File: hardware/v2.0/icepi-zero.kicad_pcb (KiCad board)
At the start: 4 copper layers, 65 x 30 mm, 208 parts, among them IC1 IS42S16160J-6BLI, IC2 LTC2256CUJ-12#PBF, IC4 LTC2622IMS8#PBF, J1 Conn_02x20_Counter_Clockwise, J2 GPDI_C_1.3, J3 USB_C_Receptacle_USB2.0_14P, J4 USB_C_Receptacle_USB2.0_14P, J5 USB_C_Receptacle_USB2.0_14P, J6 Micro_SD_Card_Det2, J7 RSP-122811-01, J8 BM04B-ACHSS-A-GAN-TFLFSN, SW1 SW_Push, SW2 SW_Push, U1 ECP5U-25F-CABGA256, U10 TPD2EUSB30A, U11 LT1993CUD-2_PBF, U12 W25Q128JVS, U13 TCR5FM50A, U2 LTC3407AEDD-2_PBF, U3 TLV62569DBV, U5 TCR5FM18A, U6 PCA9306DC1, U7 TPD2EUSB30A, U8 TPD2EUSB30A, U9 FT231XQ, Y1 SG-8018CG 50.000000MHz, Y2 SG-8018CG 25.000000MHz

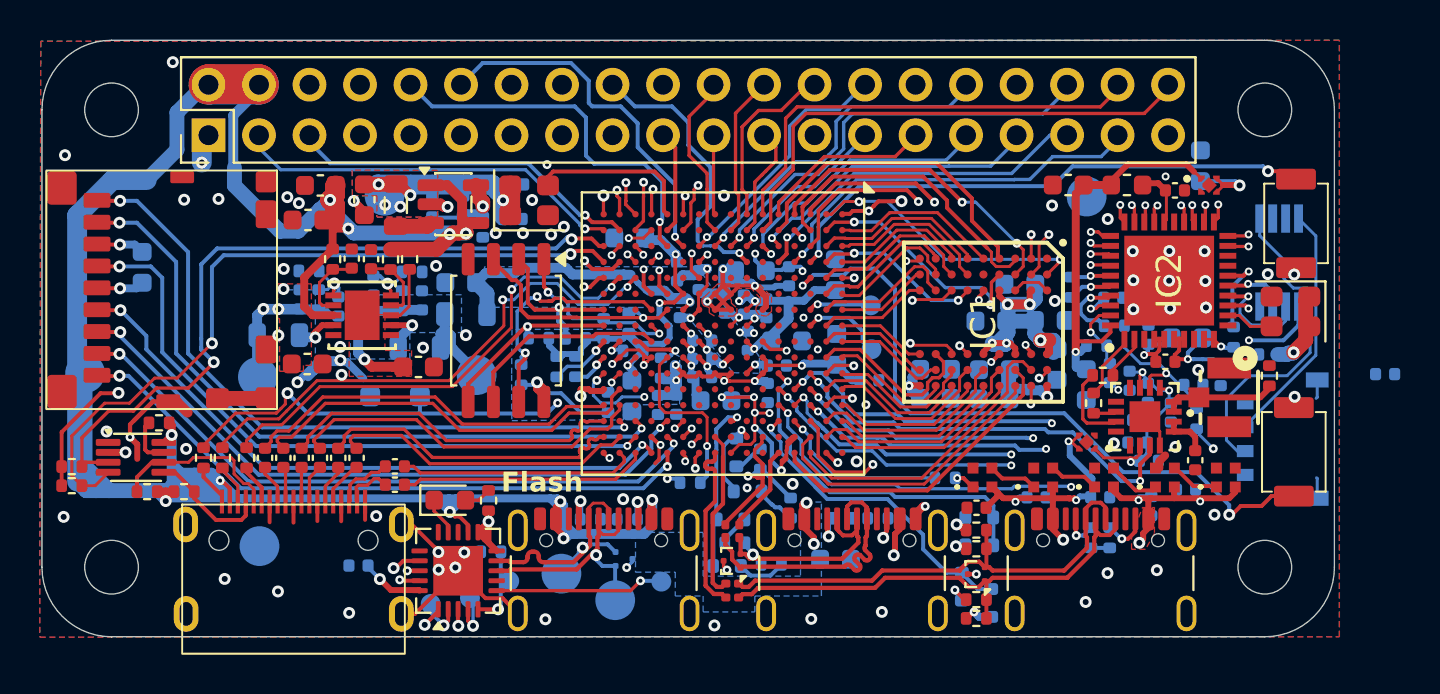
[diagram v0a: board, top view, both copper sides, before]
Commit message: DRC pass
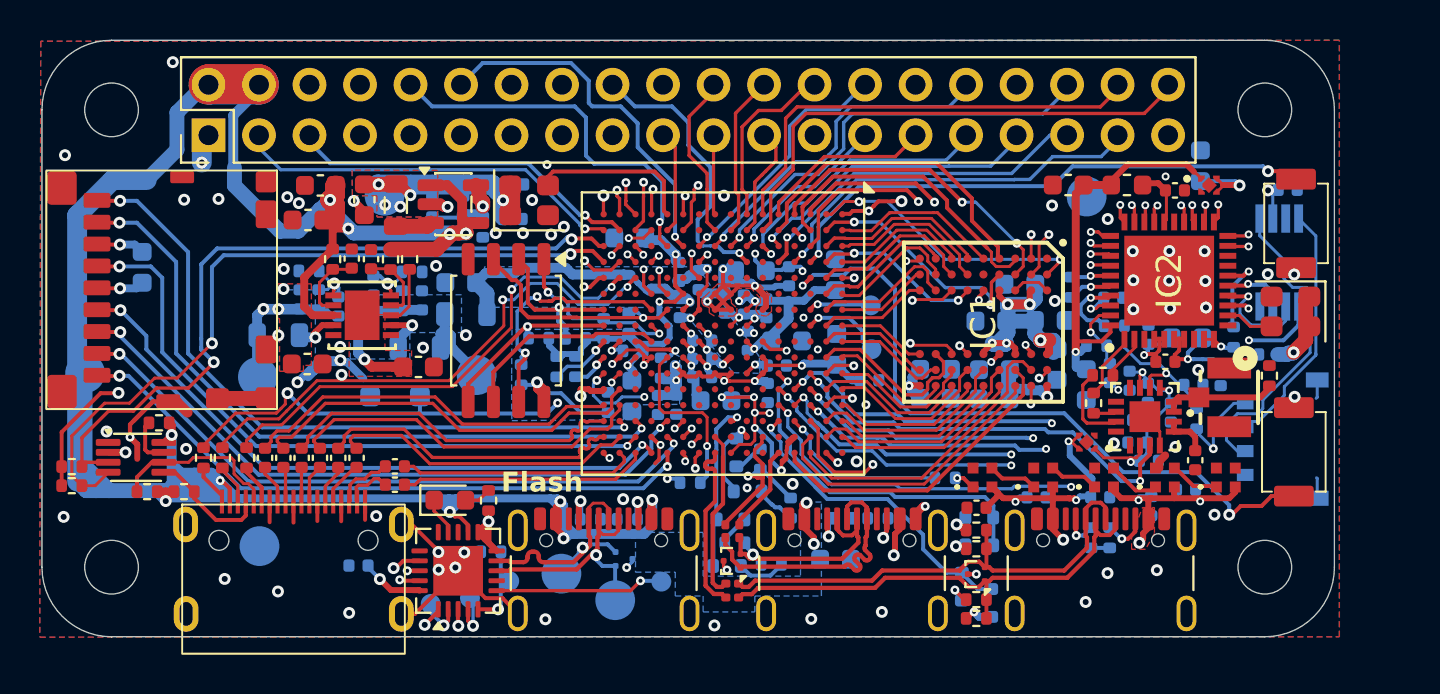
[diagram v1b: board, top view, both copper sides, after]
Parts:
- moved C82 10.5 mm to (178.4, 97.5)
- moved C25 0.10 mm to (147.8, 101.7)
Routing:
- net +3V3: track 125.3 -> 128.9 mm, vias 32 -> 33
- net /DAC/VOUT_B: track 16.6 -> 16.1 mm
